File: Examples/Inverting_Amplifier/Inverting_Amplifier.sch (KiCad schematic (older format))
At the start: 6 parts, among them X1 UA741

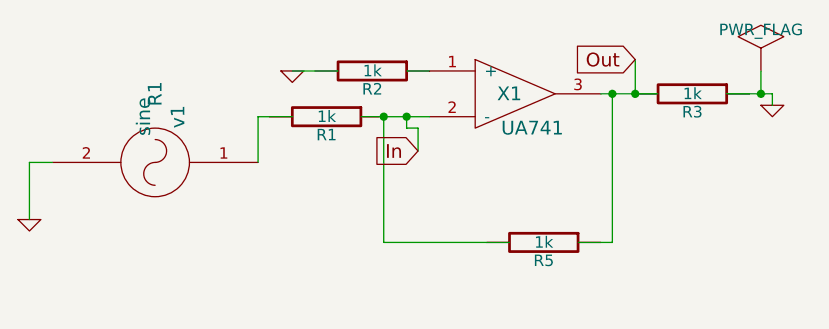
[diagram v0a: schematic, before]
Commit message: Modified Example
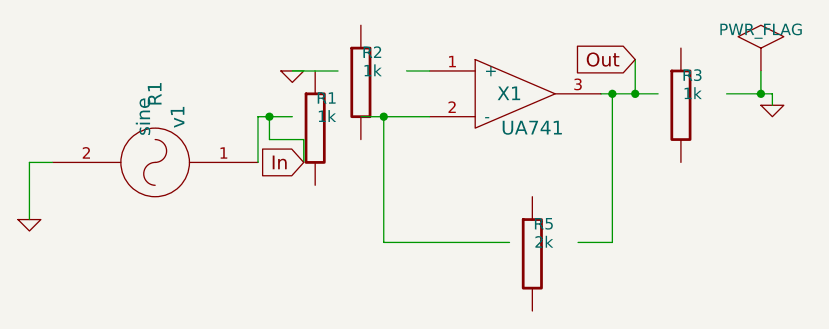
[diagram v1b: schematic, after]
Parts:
- R5: value 1k -> 2k
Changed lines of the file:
@@
 EESchema Schematic File Version 2
+LIBS:eSim_Analog
+LIBS:eSim_Devices
+LIBS:eSim_Digital
+LIBS:eSim_Hybrid
+LIBS:eSim_Miscellaneous
+LIBS:eSim_Sources
+LIBS:eSim_Subckt
+LIBS:eSim_User
+LIBS:Inverting_Amplifier-rescue
 LIBS:power
 LIBS:device
@@
 LIBS:memory
 LIBS:xilinx
-LIBS:special
 LIBS:microcontrollers
 LIBS:dsp
@@
 LIBS:contrib
 LIBS:valves
-LIBS:eSim_Analog
-LIBS:eSim_Devices
-LIBS:eSim_Digital
-LIBS:eSim_Hybrid
-LIBS:eSim_Sources
-LIBS:eSim_Subckt
+LIBS:Inverting_Amplifier-cache
 EELAYER 25 0
 EELAYER END
@@
 $EndComp
 $Comp
-L R R2
-U 1 1 558821D4
-P 5050 3300
-F 0 "R2" V 5130 3300 50  0000 C CNN
-F 1 "1k" V 5050 3300 50  0000 C CNN
-F 2 "" V 4980 3300 30  0000 C CNN
-F 3 "" H 5050 3300 30  0000 C CNN
-	1    5050 3300
-	0    1    1    0
-$EndComp
-$Comp
-L R R3
-U 1 1 558821F0
-P 6450 3400
-F 0 "R3" V 6530 3400 50  0000 C CNN
-F 1 "1k" V 6450 3400 50  0000 C CNN
-F 2 "" V 6380 3400 30  0000 C CNN
-F 3 "" H 6450 3400 30  0000 C CNN
-	1    6450 3400
-	0    1    1    0
-$EndComp
-$Comp
-L GND #PWR01
+L GND-RESCUE-Inverting_Amplifier #PWR01
 U 1 1 5588243E
 P 3550 3950
@@
 $EndComp
 $Comp
-L GND #PWR02
+L GND-RESCUE-Inverting_Amplifier #PWR02
 U 1 1 558824A7
 P 6800 3450
@@
 Text GLabel 6200 3250 0    60   Input ~ 0
 Out
-Text GLabel 5250 3650 0    60   Input ~ 0
+Text GLabel 4750 3700 0    60   Input ~ 0
 In
 $Comp
@@
 $EndComp
 $Comp
-L R R5
-U 1 1 558828E5
-P 5800 4050
-F 0 "R5" V 5880 4050 50  0000 C CNN
-F 1 "1k" V 5800 4050 50  0000 C CNN
-F 2 "" V 5730 4050 30  0000 C CNN
-F 3 "" H 5800 4050 30  0000 C CNN
-	1    5800 4050
-	0    1    1    0
-$EndComp
-$Comp
-L GND #PWR04
+L GND-RESCUE-Inverting_Amplifier #PWR04
 U 1 1 55882C4B
 P 4700 3300
@@
 	0    1    1    0
 $EndComp
-$Comp
-L R R1
-U 1 1 55882CF2
-P 4850 3500
-F 0 "R1" V 4930 3500 50  0000 C CNN
-F 1 "1k" V 4850 3500 50  0000 C CNN
-F 2 "" V 4780 3500 30  0000 C CNN
-F 3 "" H 4850 3500 30  0000 C CNN
-	1    4850 3500
-	0    1    1    0
-$EndComp
 Wire Wire Line
 	4550 3500 4550 3700
@@
 Wire Wire Line
 	3550 3700 3550 3950
-Wire Wire Line
-	5250 3650 5250 3550
-Wire Wire Line
-	5250 3550 5200 3550
-Wire Wire Line
-	5200 3550 5200 3500
-Connection ~ 5200 3500
+Connection ~ 4600 3500
 Wire Wire Line
 	6200 3250 6200 3400
@@
 Wire Wire Line
 	5000 3500 5300 3500
+$Comp
+L R R2
+U 1 1 55D44FCE
+P 5000 3350
+F 0 "R2" H 5050 3480 50  0000 C CNN
+F 1 "1k" H 5050 3400 50  0000 C CNN
+F 2 "" H 5050 3330 30  0000 C CNN
+F 3 "" V 5050 3400 30  0000 C CNN
+	1    5000 3350
+	1    0    0    -1
+$EndComp
+$Comp
+L R R1
+U 1 1 55D45007
+P 4800 3550
+F 0 "R1" H 4850 3680 50  0000 C CNN
+F 1 "1k" H 4850 3600 50  0000 C CNN
+F 2 "" H 4850 3530 30  0000 C CNN
+F 3 "" V 4850 3600 30  0000 C CNN
+	1    4800 3550
+	1    0    0    -1
+$EndComp
+$Comp
+L R R5
+U 1 1 55D450F9
+P 5750 4100
+F 0 "R5" H 5800 4230 50  0000 C CNN
+F 1 "2k" H 5800 4150 50  0000 C CNN
+F 2 "" H 5800 4080 30  0000 C CNN
+F 3 "" V 5800 4150 30  0000 C CNN
+	1    5750 4100
+	1    0    0    -1
+$EndComp
+$Comp
+L R R3
+U 1 1 55D4519D
+P 6400 3450
+F 0 "R3" H 6450 3580 50  0000 C CNN
+F 1 "1k" H 6450 3500 50  0000 C CNN
+F 2 "" H 6450 3430 30  0000 C CNN
+F 3 "" V 6450 3500 30  0000 C CNN
+	1    6400 3450
+	1    0    0    -1
+$EndComp
+Wire Wire Line
+	4600 3500 4600 3600
+Wire Wire Line
+	4600 3600 4750 3600
+Wire Wire Line
+	4750 3600 4750 3700
 $EndSCHEMATC
